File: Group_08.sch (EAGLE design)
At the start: 28 parts, among them J1 POWER_JACKPTH_LOCK, U1 +12v, U3 TCA9546ATSSOP, U4 TMUX1208

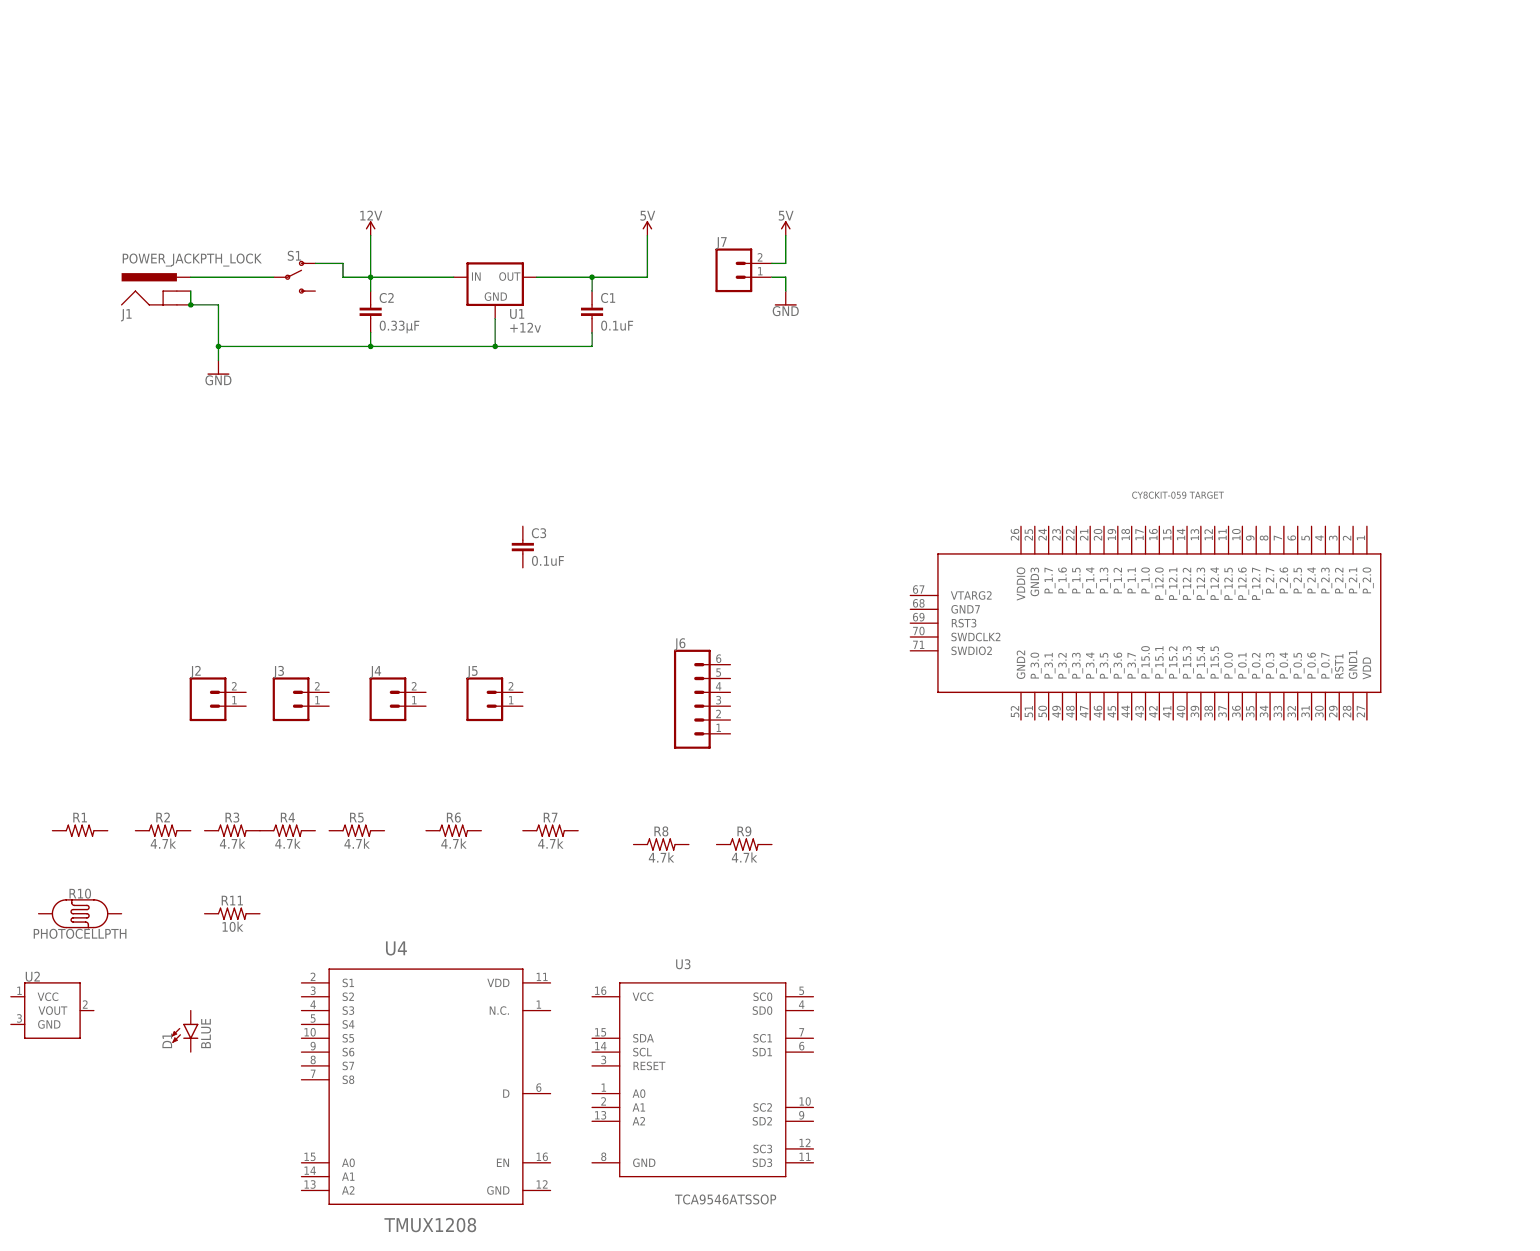
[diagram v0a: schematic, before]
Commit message: completed wiring
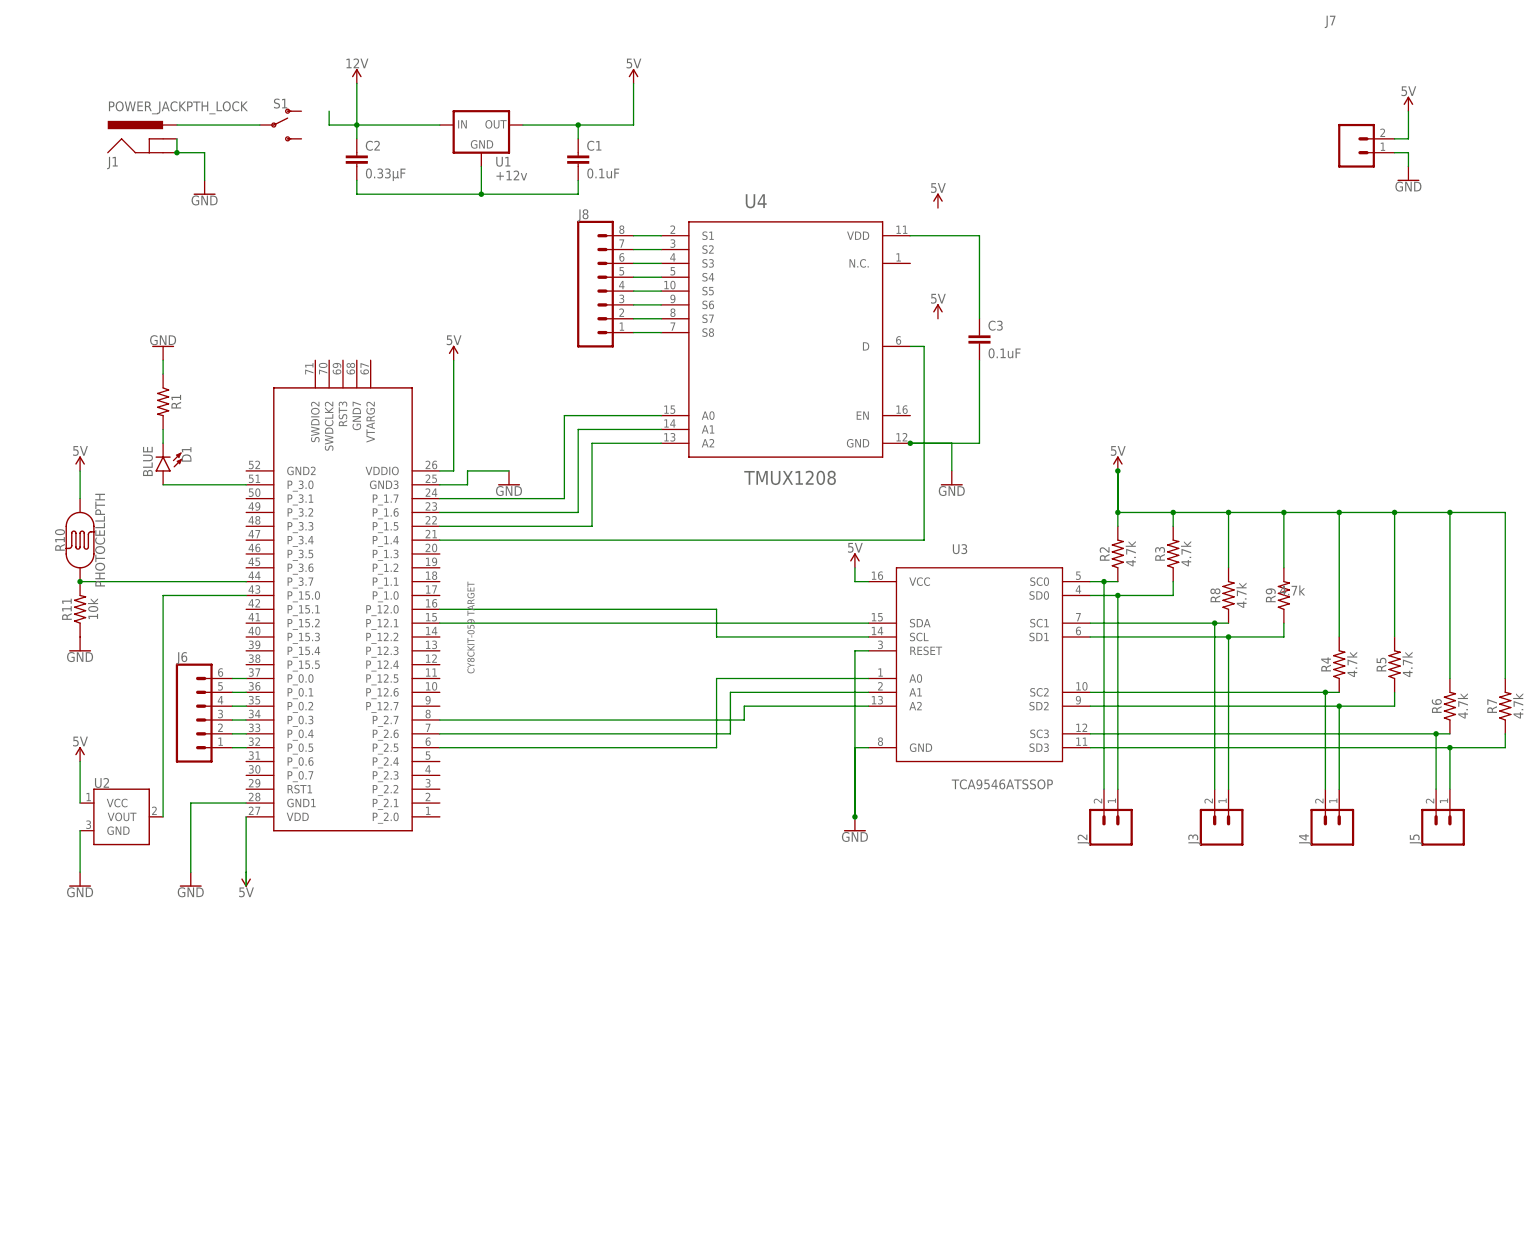
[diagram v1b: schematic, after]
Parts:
- added J8: (no value), SparkFun-Connectors:CONN_08LOCK
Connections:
- new net N$10: U$1.P_2.5, U3.A0
- new net N$11: U$1.P_2.6, U3.A1
- new net N$12: U$1.P_2.7, U3.A2
- new net N$13: U$1.P_12.0, U3.SCL
- new net N$14: U$1.P_12.1, U3.SDA
- new net N$15: C1.2, C2.2, U1.GND
- new net N$16: J6.6, U$1.P_0.0
- new net N$17: J6.5, U$1.P_0.1
- new net N$18: J6.4, U$1.P_0.2
- new net N$19: J6.3, U$1.P_0.3
- new net N$20: J6.2, U$1.P_0.4
- new net N$21: J6.1, U$1.P_0.5
- new net N$22: U$1.P_1.7, U4.A0
- new net N$23: U$1.P_1.6, U4.A1
- new net N$24: U$1.P_1.5, U4.A2
- new net N$25: U$1.P_1.4, U4.D
- new net N$26: R10.P$1, R11.2, U$1.P_3.7
- new net N$27: U$1.P_15.0, U2.VOUT
- new net N$28: D1.C, R1.2
- new net N$29: J8.8, U4.S1
- new net N$3: J2.1, R3.1, U3.SD0
- new net N$30: J8.7, U4.S2
- new net N$31: J8.6, U4.S3
- new net N$32: J8.5, U4.S4
- new net N$33: J8.4, U4.S5
- new net N$34: J8.3, U4.S6
- new net N$35: J8.2, U4.S7
- new net N$36: J8.1, U4.S8
- new net N$37: C3.1, U4.VDD
- new net N$38: D1.A, U$1.P_3.0
- new net N$4: J3.2, R8.1, U3.SC1
- new net N$5: J3.1, R9.1, U3.SD1
- new net N$6: J4.2, R4.1, U3.SC2
- new net N$7: J4.1, R5.1, U3.SD2
- new net N$8: J5.2, R6.1, U3.SC3
- new net N$9: J5.1, R7.1, U3.SD3
- net 12V: no longer S1.O
- net 5V: now also R10.P$2, R2.2, R3.2, R4.2, R5.2, R6.2, R7.2, R8.2, R9.2, U$1.VDD, U$1.VDDIO, U2.VCC, U3.VCC
- net GND: now also C3.2, R1.1, R11.1, U$1.GND1, U$1.GND3, U2.GND, U3.GND, U3.RESET, U4.GND; no longer C1.2, C2.2, U1.GND
- net N$1: now also J2.2, R2.1, U3.SC0; no longer R3.2, R4.1
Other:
- moved on the sheet: C1, C2, C3, D1, J1, J2, J3, J4, J5, J6, J7, R1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
